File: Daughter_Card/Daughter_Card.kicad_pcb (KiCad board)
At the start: 2 copper layers, 67.6 x 31.1 mm, 106 parts, among them P10 Conn_01x01_Pin, P100 Conn_01x01_Pin, P11 Conn_01x01_Pin, P12 Conn_01x01_Pin, P14 Conn_01x01_Pin, P15 Conn_01x01_Pin, P16 Conn_01x01_Pin, P17 Conn_01x01_Pin, P18 Conn_01x01_Pin, P19 Conn_01x01_Pin, P20 Conn_01x01_Pin, P21 Conn_01x01_Pin, P22 Conn_01x01_Pin, P23 Conn_01x01_Pin, P24 Conn_01x01_Pin, P25 Conn_01x01_Pin, P26 Conn_01x01_Pin, P27 Conn_01x01_Pin, P28 Conn_01x01_Pin, P29 Conn_01x01_Pin, P3 Conn_01x01_Pin, P30 Conn_01x01_Pin, P31 Conn_01x01_Pin, P32 Conn_01x01_Pin, P33 Conn_01x01_Pin, P34 Conn_01x01_Pin, P35 Conn_01x01_Pin, P36 Conn_01x01_Pin, P37 Conn_01x01_Pin, P38 Conn_01x01_Pin, P39 Conn_01x01_Pin, P4 Conn_01x01_Pin, P40 Conn_01x01_Pin, P41 Conn_01x01_Pin, P42 Conn_01x01_Pin, P43 Conn_01x01_Pin, P44 Conn_01x01_Pin, P45 Conn_01x01_Pin, P46 Conn_01x01_Pin, P47 Conn_01x01_Pin, P48 Conn_01x01_Pin, P49 Conn_01x01_Pin, P5 Conn_01x01_Pin, P50 Conn_01x01_Pin, P51 Conn_01x01_Pin, P52 Conn_01x01_Pin, P53 Conn_01x01_Pin, P54 Conn_01x01_Pin, P55 Conn_01x01_Pin, P56 Conn_01x01_Pin, P57 Conn_01x01_Pin, P58 Conn_01x01_Pin, P59 Conn_01x01_Pin, P6 Conn_01x01_Pin, P60 Conn_01x01_Pin, P61 Conn_01x01_Pin, P62 Conn_01x01_Pin, P63 Conn_01x01_Pin, P64 Conn_01x01_Pin, P65 Conn_01x01_Pin, P66 Conn_01x01_Pin, P67 Conn_01x01_Pin, P68 Conn_01x01_Pin, P69 Conn_01x01_Pin, P7 Conn_01x01_Pin, P70 Conn_01x01_Pin, P71 Conn_01x01_Pin, P72 Conn_01x01_Pin, P73 Conn_01x01_Pin, P74 Conn_01x01_Pin, P75 Conn_01x01_Pin, P76 Conn_01x01_Pin, P77 Conn_01x01_Pin, P78 Conn_01x01_Pin, P79 Conn_01x01_Pin, P8 Conn_01x01_Pin, P80 Conn_01x01_Pin, P81 Conn_01x01_Pin, P82 Conn_01x01_Pin, P83 Conn_01x01_Pin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

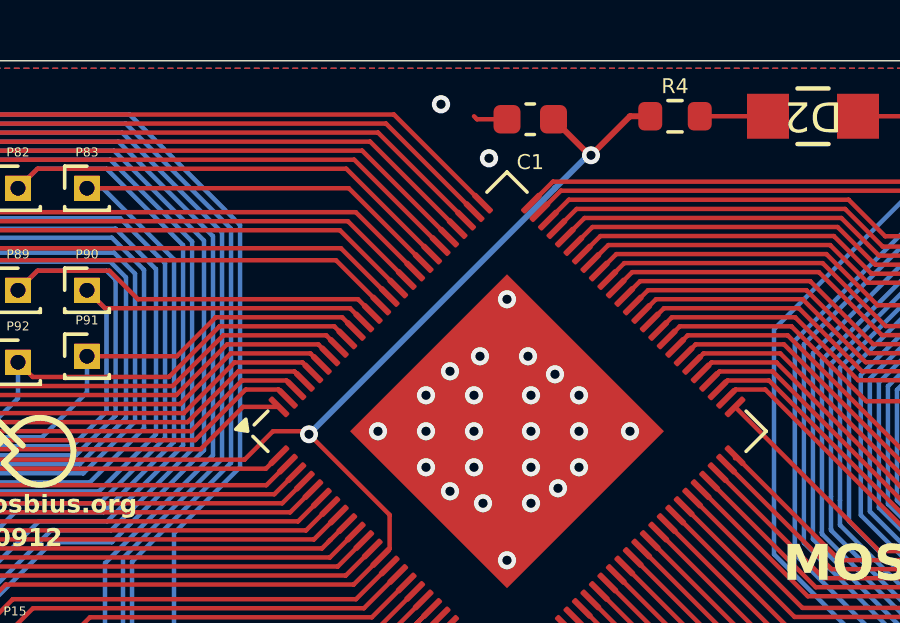
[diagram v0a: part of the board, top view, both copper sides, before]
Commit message: 0919
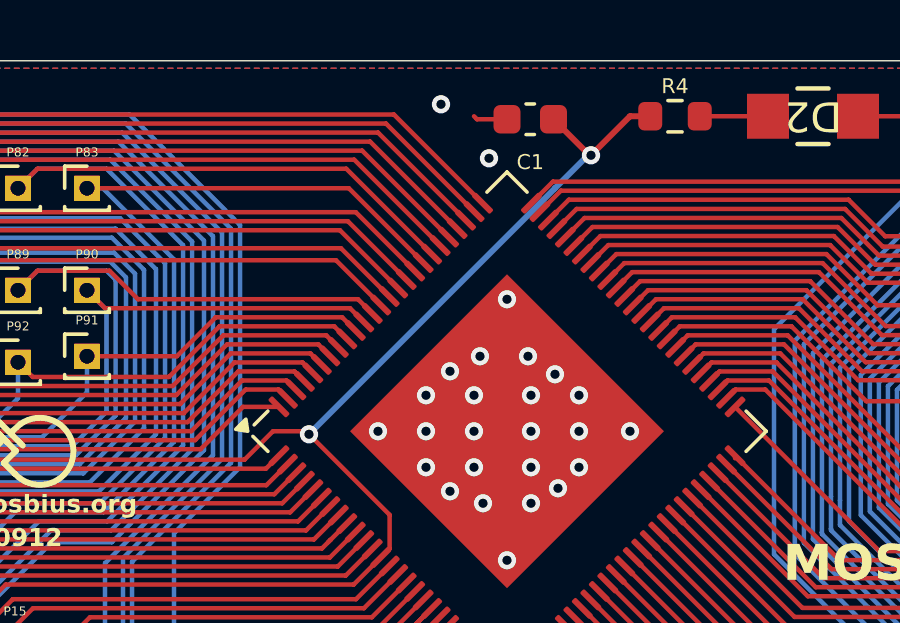
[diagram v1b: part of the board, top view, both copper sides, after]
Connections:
- MOSbius_V2 pad : (no net) -> GND
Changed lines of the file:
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@@
 			(roundrect_rratio 0.125628)
 		)
+		(pad "" smd rect
+			(at 0.53855 -0.223075 45)
+			(size 7.4 7.4)
+			(property pad_prop_heatsink)
+			(layers "F.Cu" "F.Mask")
+			(net 1 "GND")
+			(zone_connect 2)
+		)
 		(pad "" smd roundrect
 			(at 0.53855 3.270033 45)
@@
 			(pintype "bidirectional")
 		)
-		(pad "101" smd rect
-			(at 0.53855 -0.223075 45)
-			(size 7.4 7.4)
-			(property pad_prop_heatsink)
-			(layers "F.Cu" "F.Mask")
-			(zone_connect 2)
-		)
 		(embedded_fonts no)
 		(model "${KICAD9_3DMODEL_DIR}/Package_DFN_QFN.3dshapes/ArtInChip_QFN-100-1EP_12x12mm_P0.4mm_EP7.4x7.4mm.step"
@@
 	(via
 		(at 95.4 48.3)
-		(size 0.6)
-		(drill 0.3)
+		(size 0.6096)
+		(drill 0.3048)
 		(layers "F.Cu" "B.Cu")
 		(net 2)
@@
 	(via
 		(at 104.8 39)
-		(size 0.6)
-		(drill 0.3)
+		(size 0.6096)
+		(drill 0.3048)
 		(layers "F.Cu" "B.Cu")
 		(net 2)
